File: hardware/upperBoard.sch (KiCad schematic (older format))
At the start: 23 parts, among them J1 Program interface, J2 Conn_02x10_Odd_Even, Q1 MMBT3904, Q2 MMBT3904, SW1 Reset, SW2 Prog, U1 ESP-12F, U2 A2982, U3 MCP23017_SO, U4 A2982

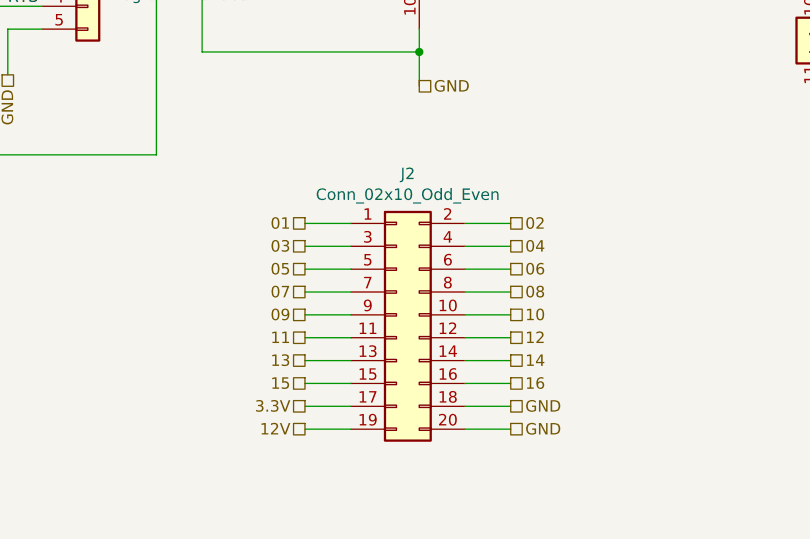
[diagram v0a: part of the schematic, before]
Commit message: continue to design lower pcb
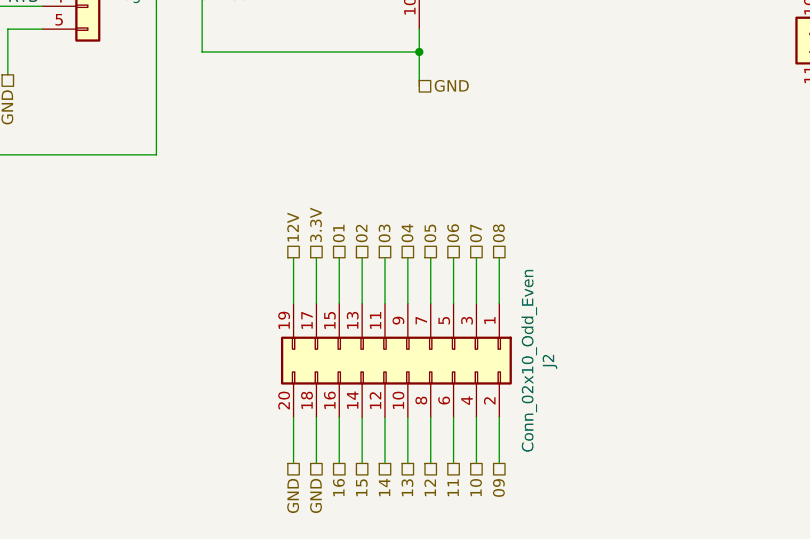
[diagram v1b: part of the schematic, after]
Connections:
- net 01: now also J2.15 (Pin_15); no longer J2.1 (Pin_1)
- net 02: now also J2.13 (Pin_13); no longer J2.2 (Pin_2)
- net 03: now also J2.11 (Pin_11); no longer J2.3 (Pin_3)
- net 04: now also J2.9 (Pin_9); no longer J2.4 (Pin_4)
- net 05: now also J2.7 (Pin_7); no longer J2.5 (Pin_5)
- net 06: now also J2.5 (Pin_5); no longer J2.6 (Pin_6)
- net 07: now also J2.3 (Pin_3); no longer J2.7 (Pin_7)
- net 08: now also J2.1 (Pin_1); no longer J2.8 (Pin_8)
- net 09: now also J2.2 (Pin_2); no longer J2.9 (Pin_9)
- net 10: now also J2.4 (Pin_4); no longer J2.10 (Pin_10)
- net 11: now also J2.6 (Pin_6); no longer J2.11 (Pin_11)
- net 12: now also J2.8 (Pin_8); no longer J2.12 (Pin_12)
- net 13: now also J2.10 (Pin_10); no longer J2.13 (Pin_13)
- net 14: now also J2.12 (Pin_12); no longer J2.14 (Pin_14)
- net 15: now also J2.14 (Pin_14); no longer J2.15 (Pin_15)
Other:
- moved on the sheet: J2
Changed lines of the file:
@@
 Wire Wire Line
 	3300 2600 4450 2600
-Text HLabel 5400 6300 0    50   UnSpc ~ 0
-3.3V
-Text HLabel 6300 6300 2    50   UnSpc ~ 0
+Text HLabel 5450 5650 1    50   UnSpc ~ 0
+3.3V
+Text HLabel 5450 6550 3    50   UnSpc ~ 0
 GND
 Text HLabel 3950 3300 3    50   UnSpc ~ 0
@@
 Text HLabel 4450 1750 1    50   UnSpc ~ 0
 3.3V
-Text HLabel 5400 6200 0    50   UnSpc ~ 0
+Text HLabel 5650 6550 3    50   UnSpc ~ 0
 15
-Text HLabel 5400 6100 0    50   UnSpc ~ 0
+Text HLabel 5850 6550 3    50   UnSpc ~ 0
 13
-Text HLabel 5400 6000 0    50   UnSpc ~ 0
+Text HLabel 6050 6550 3    50   UnSpc ~ 0
 11
-Text HLabel 5400 5900 0    50   UnSpc ~ 0
+Text HLabel 6250 6550 3    50   UnSpc ~ 0
 09
-Text HLabel 5400 5800 0    50   UnSpc ~ 0
+Text HLabel 6150 5650 1    50   UnSpc ~ 0
 07
-Text HLabel 5400 5700 0    50   UnSpc ~ 0
+Text HLabel 5950 5650 1    50   UnSpc ~ 0
 05
-Text HLabel 5400 5600 0    50   UnSpc ~ 0
+Text HLabel 5750 5650 1    50   UnSpc ~ 0
 03
-Text HLabel 5400 5500 0    50   UnSpc ~ 0
+Text HLabel 5550 5650 1    50   UnSpc ~ 0
 01
-Text HLabel 6300 6200 2    50   UnSpc ~ 0
+Text HLabel 5550 6550 3    50   UnSpc ~ 0
 16
-Text HLabel 6300 6100 2    50   UnSpc ~ 0
+Text HLabel 5750 6550 3    50   UnSpc ~ 0
 14
-Text HLabel 6300 6000 2    50   UnSpc ~ 0
+Text HLabel 5950 6550 3    50   UnSpc ~ 0
 12
-Text HLabel 6300 5900 2    50   UnSpc ~ 0
+Text HLabel 6150 6550 3    50   UnSpc ~ 0
 10
-Text HLabel 6300 5800 2    50   UnSpc ~ 0
+Text HLabel 6250 5650 1    50   UnSpc ~ 0
 08
-Text HLabel 6300 5700 2    50   UnSpc ~ 0
+Text HLabel 6050 5650 1    50   UnSpc ~ 0
 06
-Text HLabel 6300 5600 2    50   UnSpc ~ 0
+Text HLabel 5850 5650 1    50   UnSpc ~ 0
 04
-Text HLabel 6300 5500 2    50   UnSpc ~ 0
+Text HLabel 5650 5650 1    50   UnSpc ~ 0
 02
 Wire Wire Line
-	5400 5500 5600 5500
-Wire Wire Line
-	5600 5600 5400 5600
-Wire Wire Line
-	5400 5700 5600 5700
-Wire Wire Line
-	5600 5800 5400 5800
-Wire Wire Line
-	5400 5900 5600 5900
-Wire Wire Line
-	5600 6000 5400 6000
-Wire Wire Line
-	5600 6300 5400 6300
-Wire Wire Line
-	6100 5500 6300 5500
-Wire Wire Line
-	6100 5600 6300 5600
-Wire Wire Line
-	6300 5700 6100 5700
-Wire Wire Line
-	6300 5800 6100 5800
-Wire Wire Line
-	6300 5900 6100 5900
-Wire Wire Line
-	6300 6000 6100 6000
-Wire Wire Line
-	6300 6100 6100 6100
-Wire Wire Line
-	6300 6200 6100 6200
+	6250 5650 6250 5850
+Wire Wire Line
+	6150 5850 6150 5650
+Wire Wire Line
+	6050 5650 6050 5850
+Wire Wire Line
+	5950 5850 5950 5650
+Wire Wire Line
+	5850 5650 5850 5850
+Wire Wire Line
+	5750 5850 5750 5650
+Wire Wire Line
+	5450 5850 5450 5650
+Wire Wire Line
+	6250 6350 6250 6550
+Wire Wire Line
+	6150 6350 6150 6550
+Wire Wire Line
+	6050 6550 6050 6350
+Wire Wire Line
+	5950 6550 5950 6350
+Wire Wire Line
+	5850 6550 5850 6350
+Wire Wire Line
+	5750 6550 5750 6350
+Wire Wire Line
+	5650 6550 5650 6350
+Wire Wire Line
+	5550 6550 5550 6350
 Text HLabel 9600 1900 2    50   UnSpc ~ 0
 16
 Wire Wire Line
-	5600 6100 5400 6100
-Wire Wire Line
-	5600 6200 5400 6200
-Wire Wire Line
-	6100 6300 6300 6300
+	5650 5850 5650 5650
+Wire Wire Line
+	5550 5850 5550 5650
+Wire Wire Line
+	5450 6350 5450 6550
 $Comp
 L LED:HDSP-4830_2 BAR1
@@
 L Connector_Generic:Conn_02x10_Odd_Even J2
 U 1 1 5DAC3666
-P 5800 5900
-F 0 "J2" H 5850 6517 50  0000 C CNN
-F 1 "Conn_02x10_Odd_Even" H 5850 6426 50  0000 C CNN
-F 2 "Connector_PinHeader_2.54mm:PinHeader_2x10_P2.54mm_Vertical" H 5800 5900 50  0001 C CNN
-F 3 "~" H 5800 5900 50  0001 C CNN
-	1    5800 5900
-	1    0    0    -1
-$EndComp
-Text HLabel 6300 6400 2    50   UnSpc ~ 0
-GND
-Wire Wire Line
-	6300 6400 6100 6400
-Text HLabel 5400 6400 0    50   UnSpc ~ 0
+P 5850 6050
+F 0 "J2" H 5900 6667 50  0000 C CNN
+F 1 "Conn_02x10_Odd_Even" H 5900 6576 50  0000 C CNN
+F 2 "Connector_PinHeader_2.54mm:PinHeader_2x10_P2.54mm_Vertical" H 5850 6050 50  0001 C CNN
+F 3 "~" H 5850 6050 50  0001 C CNN
+	1    5850 6050
+	0    1    1    0
+$EndComp
+Text HLabel 5350 6550 3    50   UnSpc ~ 0
+GND
+Wire Wire Line
+	5350 6550 5350 6350
+Text HLabel 5350 5650 1    50   UnSpc ~ 0
 12V
 Wire Wire Line
-	5600 6400 5400 6400
+	5350 5850 5350 5650
 Text HLabel 9050 850  2    50   UnSpc ~ 0
 12V

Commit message: move on to 16A relays
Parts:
- BAR1: footprint Package_DIP:DIP-20_W7.62mm_LongPads -> Package_DIP:DIP-20_W7.62mm_Socket_LongPads
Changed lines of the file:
@@
 F 0 "BAR1" V 8104 5230 50  0000 L CNN
 F 1 "HDSP-4830_2" V 8195 5230 50  0000 L CNN
-F 2 "Package_DIP:DIP-20_W7.62mm_LongPads" H 8150 3900 50  0001 C CNN
+F 2 "Package_DIP:DIP-20_W7.62mm_Socket_LongPads" H 8150 3900 50  0001 C CNN
 F 3 "https://docs.broadcom.com/docs/AV02-1798EN" H 6150 4900 50  0001 C CNN
 	1    8150 4700
